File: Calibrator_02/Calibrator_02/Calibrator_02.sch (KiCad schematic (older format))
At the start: 30 parts, among them J1 Conn_01x04, J2 DB9_Female_MountingHoles, J3 Conn_Coaxial, J4 Conn_01x01_Female, J5 Conn_01x01_Female, J6 Conn_01x04, M1 AW9523BTQR, U1 KAQY214STLD, U2 KAQY214STLD, U3 KAQY214STLD, U4 KAQY214STLD, U5 KAQY214STLD, U6 KAQY214STLD, U7 KAQY214STLD, U8 KAQY214STLD

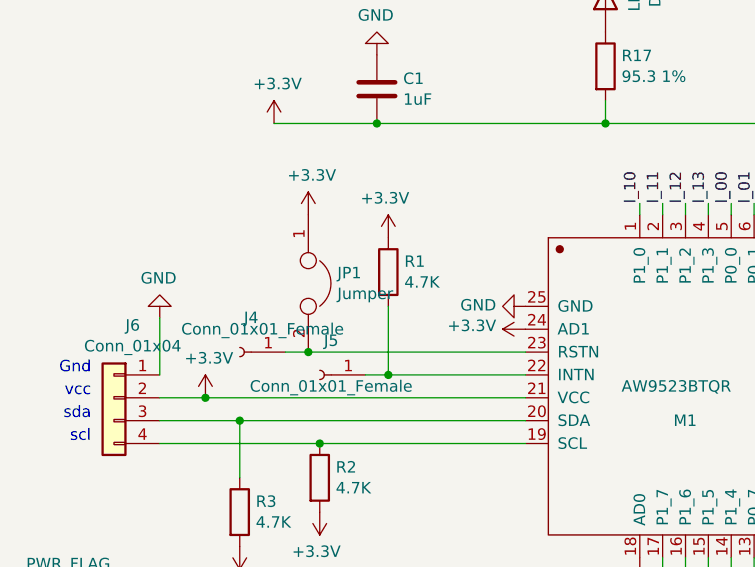
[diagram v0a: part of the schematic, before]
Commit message: Update
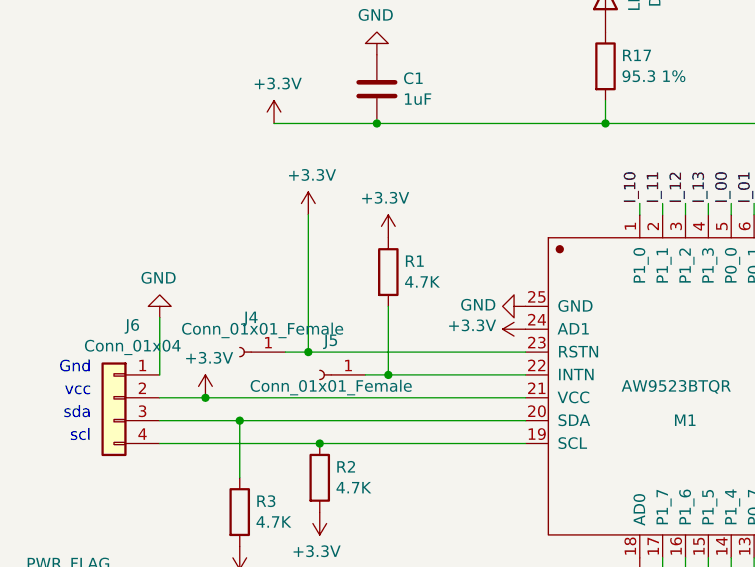
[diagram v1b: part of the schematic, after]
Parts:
- removed JP1: Jumper, Jumper:SolderJumper-2_P1.3mm_Open_RoundedPad1.0x1.5mm, symbol Device:Jumper
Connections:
- net +3V3: now also J4.1 (Pin_1), M1.23 (RSTN)
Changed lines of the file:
@@
 Wire Wire Line
 	9050 2900 9350 2900
-Wire Wire Line
-	1700 6500 1800 6500
-$Comp
-L Device:Jumper JP1
-U 1 1 627E9ED5
-P 1800 6200
-F 0 "JP1" V 1754 6327 50  0000 L CNN
-F 1 "Jumper" V 1845 6327 50  0000 L CNN
-F 2 "Jumper:SolderJumper-2_P1.3mm_Open_RoundedPad1.0x1.5mm" H 1800 6200 50  0001 C CNN
-F 3 "~" H 1800 6200 50  0001 C CNN
-	1    1800 6200
-	0    1    1    0
-$EndComp
-Connection ~ 1800 6500
-Wire Wire Line
-	1800 6500 2750 6500
 $Comp
 L power:+3.3V #PWR09
@@
 Wire Wire Line
 	3700 700  3700 1050
+Wire Wire Line
+	1700 6500 1800 6500
+Wire Wire Line
+	1800 5900 1800 6500
+Connection ~ 1800 6500
+Wire Wire Line
+	1800 6500 2750 6500
 $EndSCHEMATC
